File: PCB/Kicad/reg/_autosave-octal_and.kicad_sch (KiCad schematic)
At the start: 4 parts, among them U91 74LS08, U92 74LS08

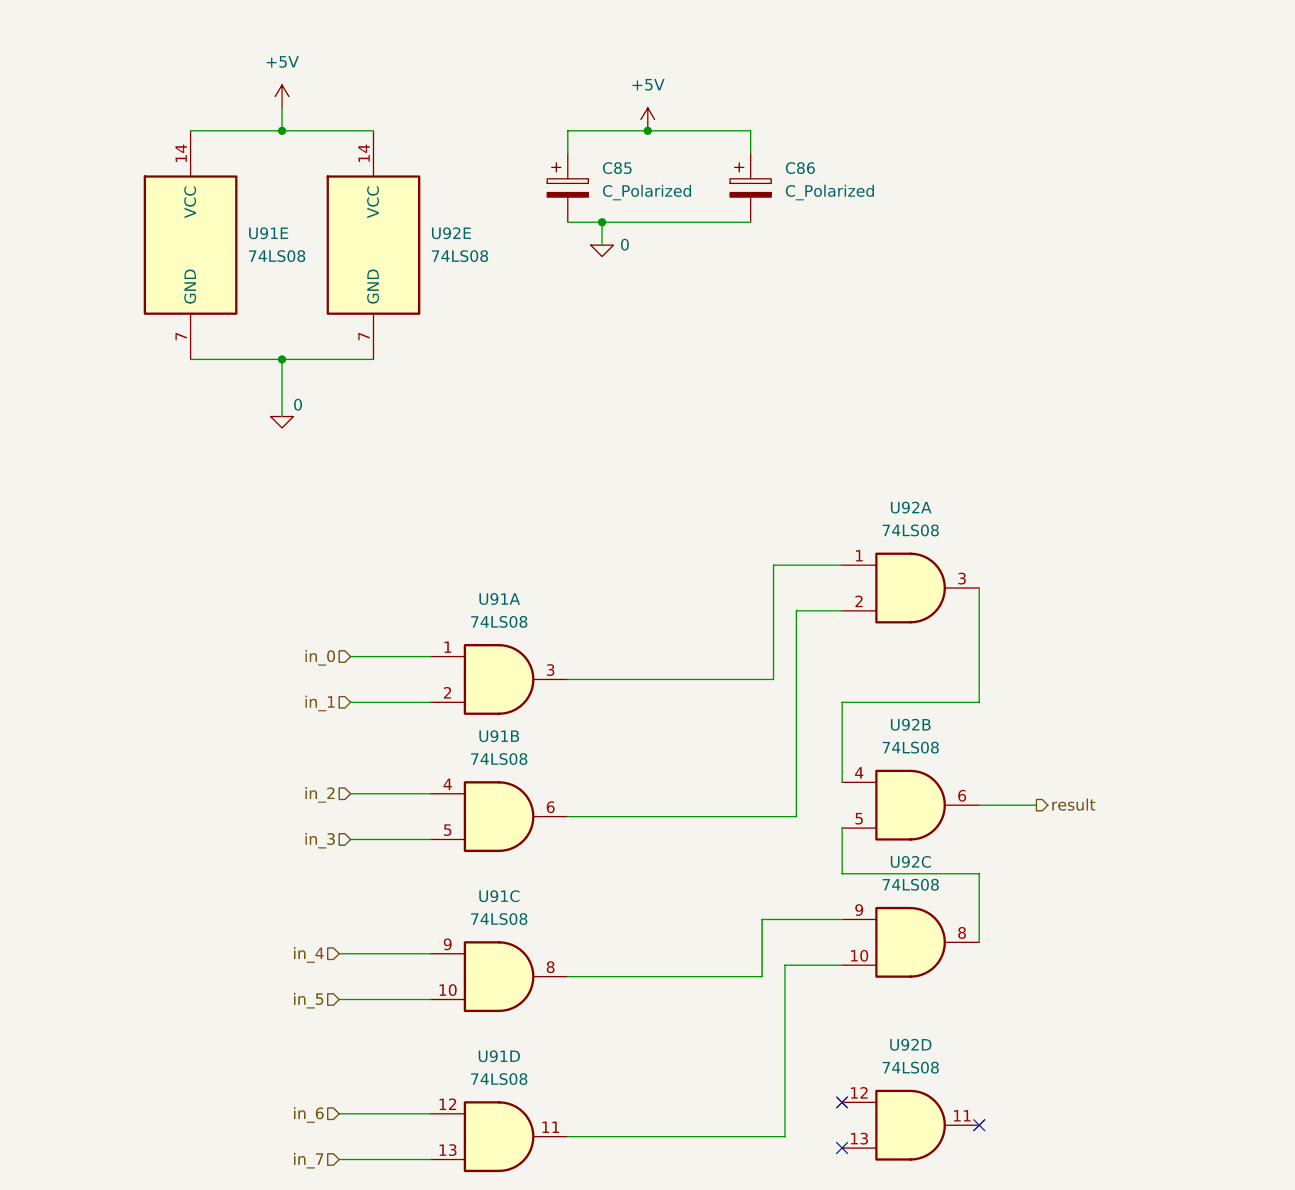
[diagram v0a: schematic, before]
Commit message: VCC
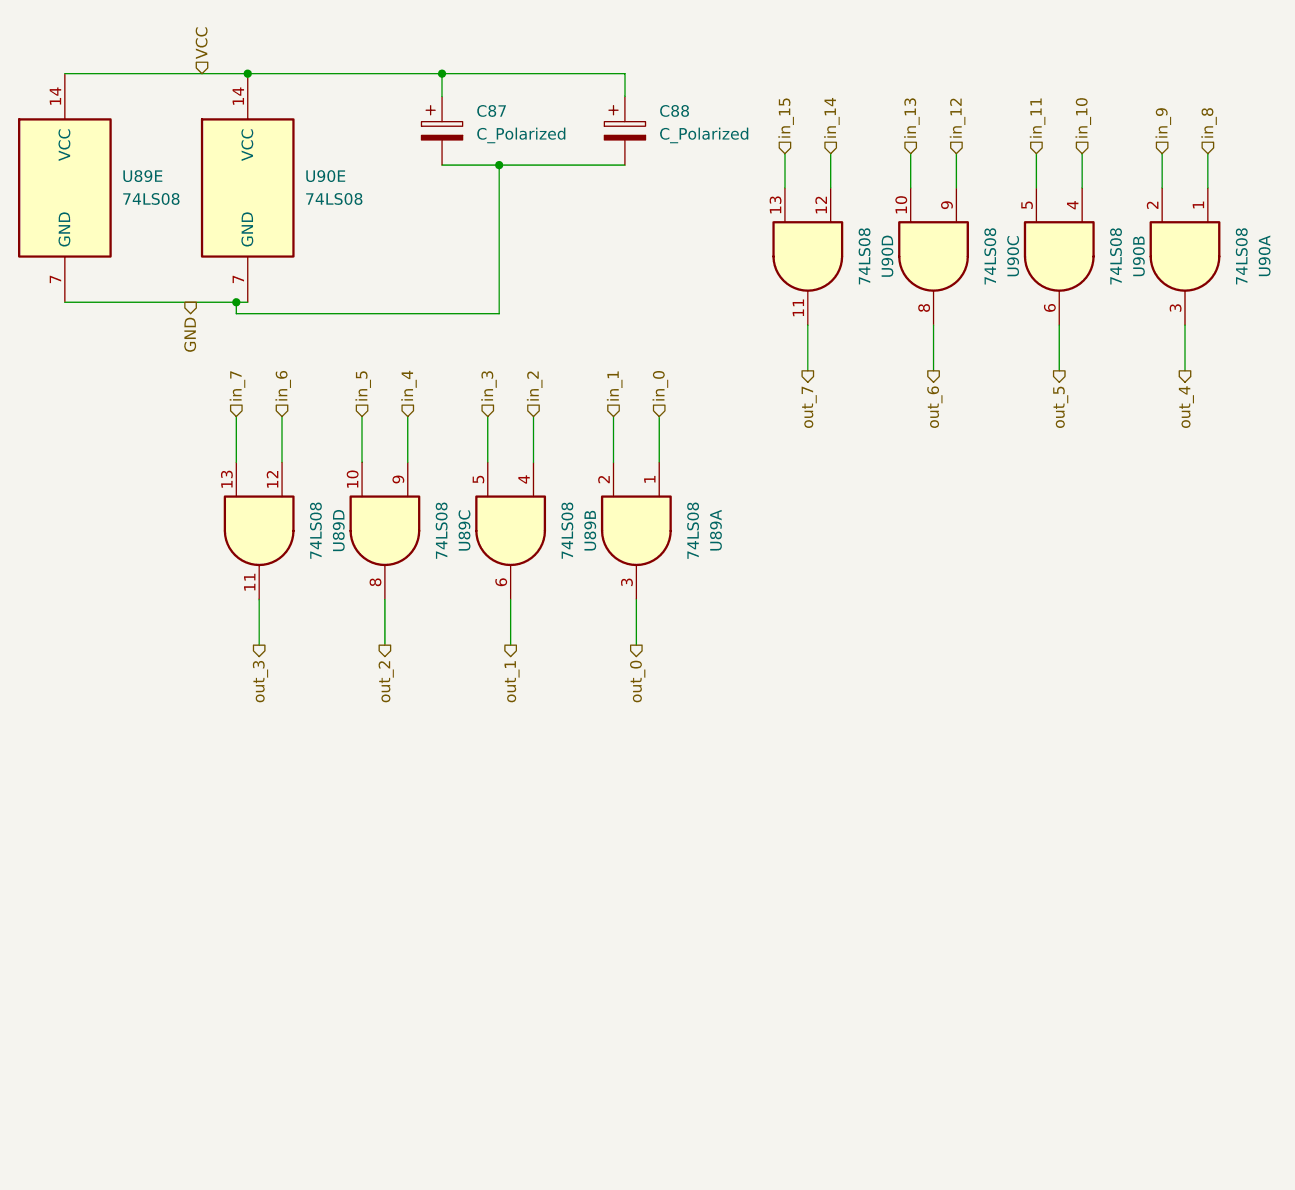
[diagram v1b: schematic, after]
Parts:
- removed C85, C86: C_Polarized, Capacitor_SMD:CP_Elec_4x3, symbol Device:C_Polarized
- removed U91: 74LS08, Package_DIP:DIP-14_W7.62mm_SMDSocket_SmallPads, symbol 74xx:74LS08
- removed U92: 74LS08, Package_DIP:DIP-20_W7.62mm_SMDSocket_SmallPads, symbol 74xx:74LS08
- added C87, C88: C_Polarized, Capacitor_SMD:CP_Elec_4x3, symbol Device:C_Polarized
- added U89: 74LS08, Package_DIP:DIP-14_W7.62mm_SMDSocket_SmallPads, symbol 74xx:74LS08
- added U90: 74LS08, Package_DIP:DIP-20_W7.62mm_SMDSocket_SmallPads, symbol 74xx:74LS08
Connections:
- net in_0: now also U89.1
- net in_1: now also U89.2
- net in_2: now also U89.4
- net in_3: now also U89.5
- net in_4: now also U89.9
- net in_5: now also U89.10
- net in_6: now also U89.12
- net in_7: now also U89.13
- new net GND: C87.2, C88.2, U89.7 (GND), U90.7 (GND)
- new net VCC: C87.1, C88.1, U89.14 (VCC), U90.14 (VCC)
- new net in_10: U90.4
- new net in_11: U90.5
- new net in_12: U90.9
- new net in_13: U90.10
- new net in_14: U90.12
- new net in_15: U90.13
- new net in_8: U90.1
- new net in_9: U90.2
- new net out_0: U89.3
- new net out_1: U89.6
- new net out_2: U89.8
- new net out_3: U89.11
- new net out_4: U90.3
- new net out_5: U90.6
- new net out_6: U90.8
- new net out_7: U90.11
- no-connect marks 3 -> 0
